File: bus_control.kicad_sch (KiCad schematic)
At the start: 12 parts, among them U24 74LS138, U3 74LS688 OR 74F521, U40 74LS138, U41 74LS00, U42 74LS08, U45 74LS138

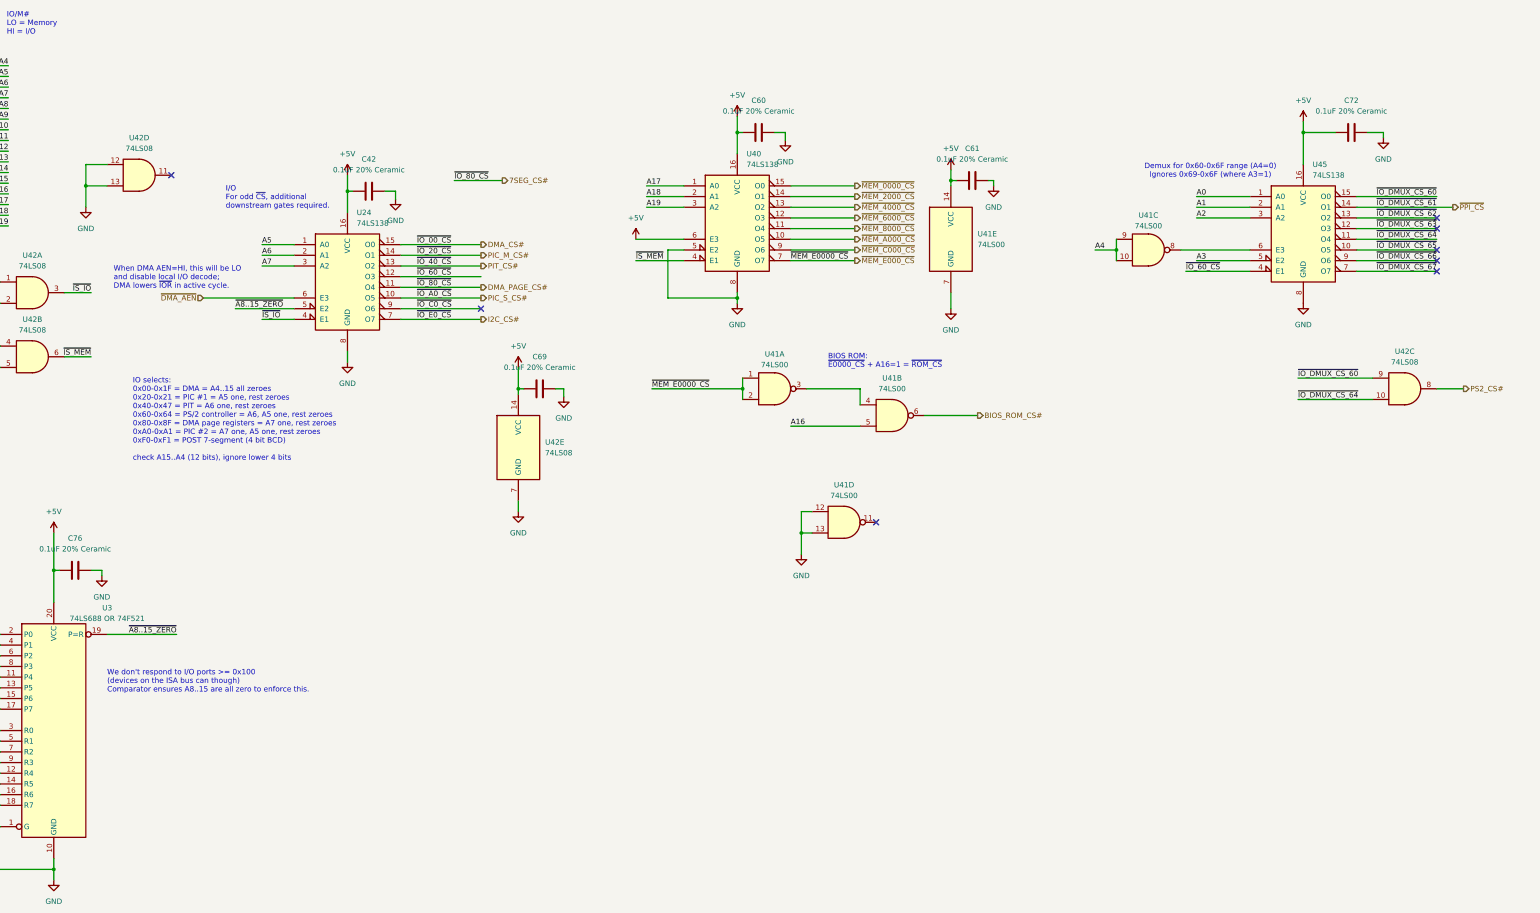
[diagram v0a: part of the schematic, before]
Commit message: no more SMT for isa_i2c, tweak motherboard multiplex logic, handful of other tweaks
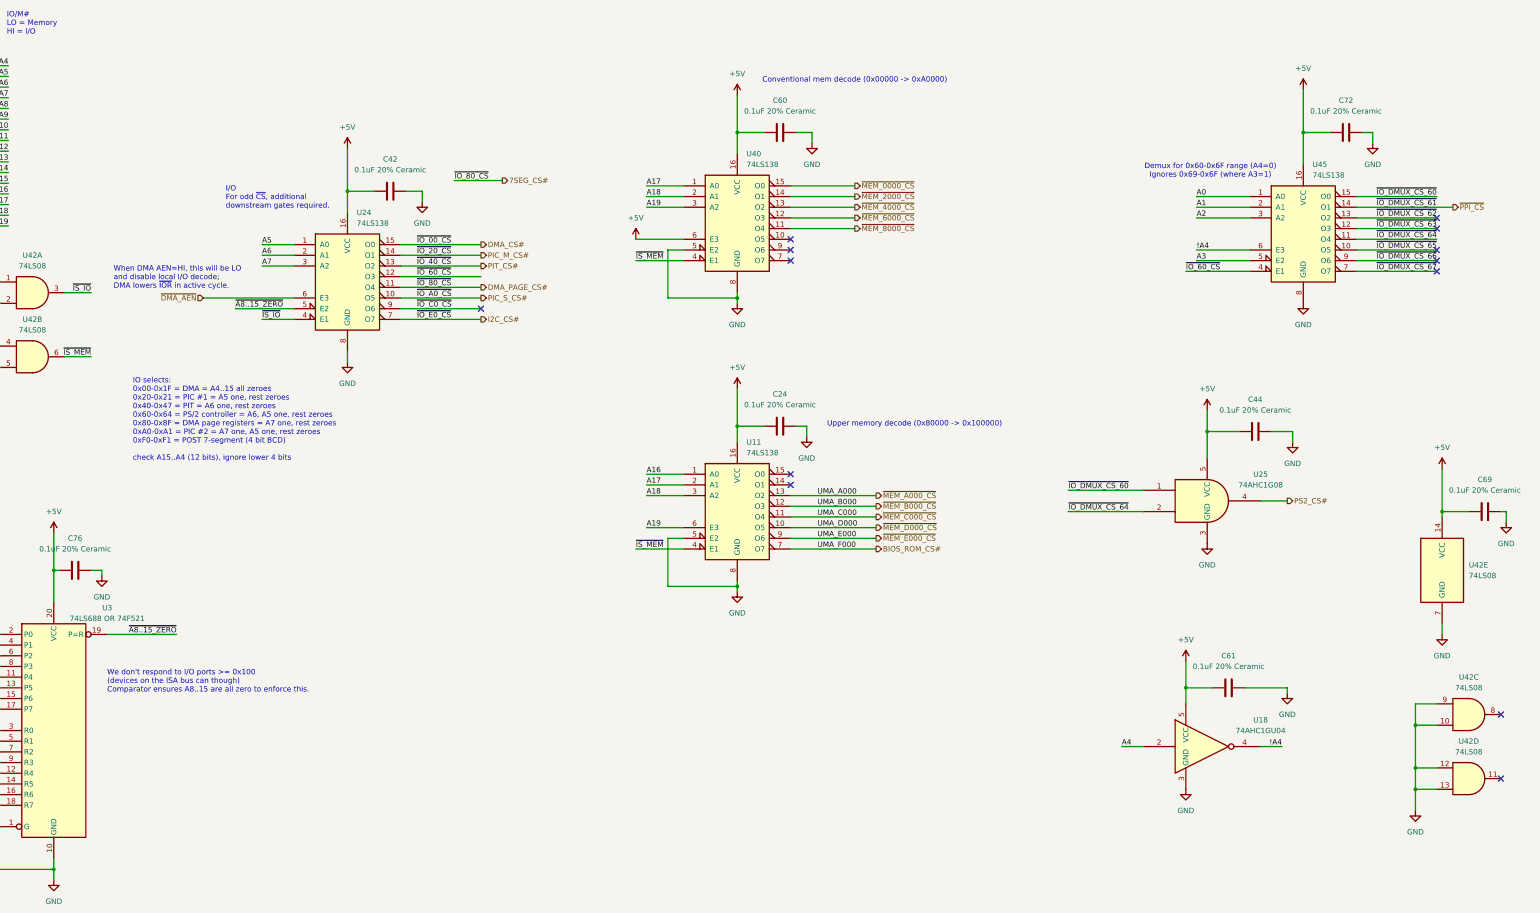
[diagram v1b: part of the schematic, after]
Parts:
- removed U41: 74LS00, Package_DIP:DIP-14_W7.62mm_Socket, symbol 74xx:74LS00
- added C24, C44: 0.1uF 20% Ceramic, Capacitor_SMD:C_0805_2012Metric, symbol Device:C
- added U11: 74LS138, Package_DIP:DIP-16_W7.62mm_Socket, symbol 74xx:74LS138
- added U18: 74AHC1GU04, Package_TO_SOT_SMD:SOT-23-5, symbol 74xGxx:74AHC1GU04
- added U25: 74AHC1G08, Package_TO_SOT_SMD:SOT-23-5, symbol 74xGxx:74AHC1G08
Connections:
- net +5V: now also C24.1, C44.1, U11.16 (VCC), U18.5 (VCC), U25.5 (VCC)
- net A16: now also U11.1 (A0)
- net A17: now also U11.2 (A1)
- net A18: now also U11.3 (A2)
- net A19: now also U11.6 (E3)
- net A4: now also U18.2
- net BIOS_ROM_CS#: now also U11.7 (O7)
- net GND: now also U42.10, U42.9, C24.2, C44.2, U11.5 (E2), U11.8 (GND), U18.3 (GND), U25.3 (GND)
- net PS2_CS#: now also U25.4; no longer U42.8
- net ~{IO_DMUX_CS_60}: now also U25.1; no longer U42.9
- net ~{IO_DMUX_CS_64}: now also U25.2; no longer U42.10
- net ~{IS_MEM}: now also U11.4 (E1)
- net ~{MEM_A000_CS}: now also U11.13 (O2); no longer U40.10 (O5)
- net ~{MEM_C000_CS}: now also U11.11 (O4); no longer U40.9 (O6)
- net ~{MEM_E000_CS}: now also U11.9 (O6); no longer U40.7 (O7)
- net !A4: now reaches U45.6 (E3)
- net !A4: now also U18.4
- new net ~{MEM_B000_CS}: U11.12 (O3)
- new net ~{MEM_D000_CS}: U11.10 (O5)
- no-connect marks 8 -> 13
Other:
- note added: "Conventional mem decode (0x00000 -> 0xA0000)"
- note added: "Upper memory decode (0x80000 -> 0x100000)"
- note removed: "BIOS ROM: ~{E0000_CS} + A16=1 = ~{ROM_CS}"
- moved on the sheet: C42, C60, C61, C69, C72, U42C, U42D, U42E
